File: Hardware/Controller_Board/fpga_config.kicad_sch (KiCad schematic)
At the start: 26 parts, among them SW301 Reset, U301 IS25LP256D, U302 XC7A35T-CSG324, Y301 12MHz

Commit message: Commit before upgrading to KiCad 10.0
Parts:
- removed unit 3 of U302
- removed unit 7 of U302
- removed unit 4 of U302
- removed unit 6 of U302
- renumbered U302 to U201
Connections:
- net 12MHZ_CLK: now also U201.C10 (IO_L13N_T2_MRCC_16)
- net at TP305.1: now also U201.D9 (IO_L6N_T0_VREF_16)
- net at U201.A8 (IO_L12N_T1_MRCC_16): now also TP301.1
- net at U201.B8 (IO_L12P_T1_MRCC_16): now also TP302.1
- net at U201.B9 (IO_L11N_T1_SRCC_16): now also TP303.1
- net at U201.C9 (IO_L11P_T1_SRCC_16): now also TP304.1
- no-connect marks 2 -> 4
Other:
- note removed: "Connect to MRCC!!!!!!"
- moved on the sheet: TP301, TP302, TP303, TP304, TP305, U201E

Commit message: Advanced PCB design: Routed FTDIs + SPI Flash
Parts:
- R303, R304, R305, R306, Re301, Re302: footprint Resistor_SMD:R_0402_1005Metric -> Resistor_SMD:R_0201_0603Metric
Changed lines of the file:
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@@
 			)
 		)
-		(property "Footprint" "Resistor_SMD:R_0402_1005Metric"
+		(property "Footprint" "Resistor_SMD:R_0201_0603Metric"
 			(at 115.57 75.438 90)
 			(hide yes)
@@
 			)
 		)
-		(property "Footprint" "Resistor_SMD:R_0402_1005Metric"
+		(property "Footprint" "Resistor_SMD:R_0201_0603Metric"
 			(at 115.57 70.358 90)
 			(hide yes)
@@
 			)
 		)
-		(property "Footprint" "Resistor_SMD:R_0402_1005Metric"
+		(property "Footprint" "Resistor_SMD:R_0201_0603Metric"
 			(at 60.96 62.738 90)
 			(hide yes)
@@
 			)
 		)
-		(property "Footprint" "Resistor_SMD:R_0402_1005Metric"
+		(property "Footprint" "Resistor_SMD:R_0201_0603Metric"
 			(at 115.57 72.898 90)
 			(hide yes)
@@
 			)
 		)
-		(property "Footprint" "Resistor_SMD:R_0402_1005Metric"
+		(property "Footprint" "Resistor_SMD:R_0201_0603Metric"
 			(at 60.96 55.118 90)
 			(hide yes)
@@
 			)
 		)
-		(property "Footprint" "Resistor_SMD:R_0402_1005Metric"
+		(property "Footprint" "Resistor_SMD:R_0201_0603Metric"
 			(at 122.428 86.36 90)
 			(hide yes)

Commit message: Advanced PCB design - Routed FTDI chips + USB HUB
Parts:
- U301: footprint Package_SON:WSON-8-1EP_8x6mm_P1.27mm_EP3.4x4.3mm -> Custom_VoxLink_Footprints:WSON-8-1EP_8.0x6.0mm_P1.27mm_EP4.7x4.6mm
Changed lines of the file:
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@@
 			)
 		)
-		(property "Footprint" "Package_SON:WSON-8-1EP_8x6mm_P1.27mm_EP3.4x4.3mm"
+		(property "Footprint" "Custom_VoxLink_Footprints:WSON-8-1EP_8.0x6.0mm_P1.27mm_EP4.7x4.6mm"
 			(at 161.29 104.14 0)
 			(hide yes)

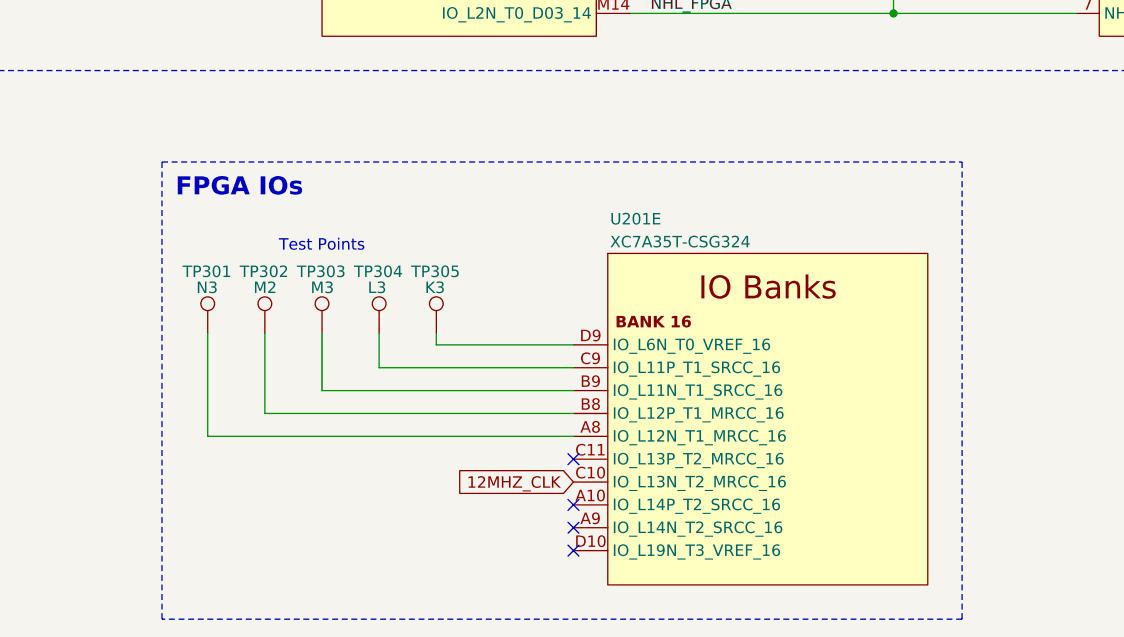
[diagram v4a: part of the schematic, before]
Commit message: Advanced PCB design: Advanced power routing
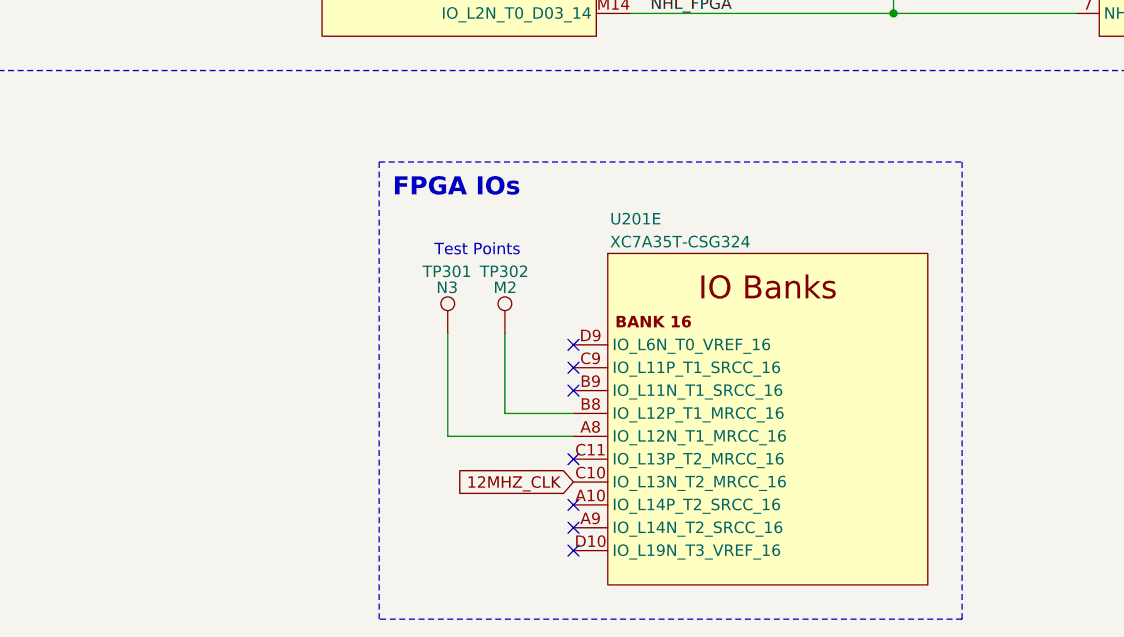
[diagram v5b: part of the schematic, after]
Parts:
- removed TP303: M3, TestPoint:TestPoint_Pad_D1.0mm, symbol Connector:TestPoint
- removed TP304: L3, TestPoint:TestPoint_Pad_D1.0mm, symbol Connector:TestPoint
- removed TP305: K3, TestPoint:TestPoint_Pad_D1.0mm, symbol Connector:TestPoint
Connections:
- no-connect marks 4 -> 7
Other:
- moved on the sheet: TP301, TP302
